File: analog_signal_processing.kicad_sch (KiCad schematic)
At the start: 62 parts, among them U3 PT2399, U4 CD4066BE, U5 PT2399, U8 TL072, U9 TL072

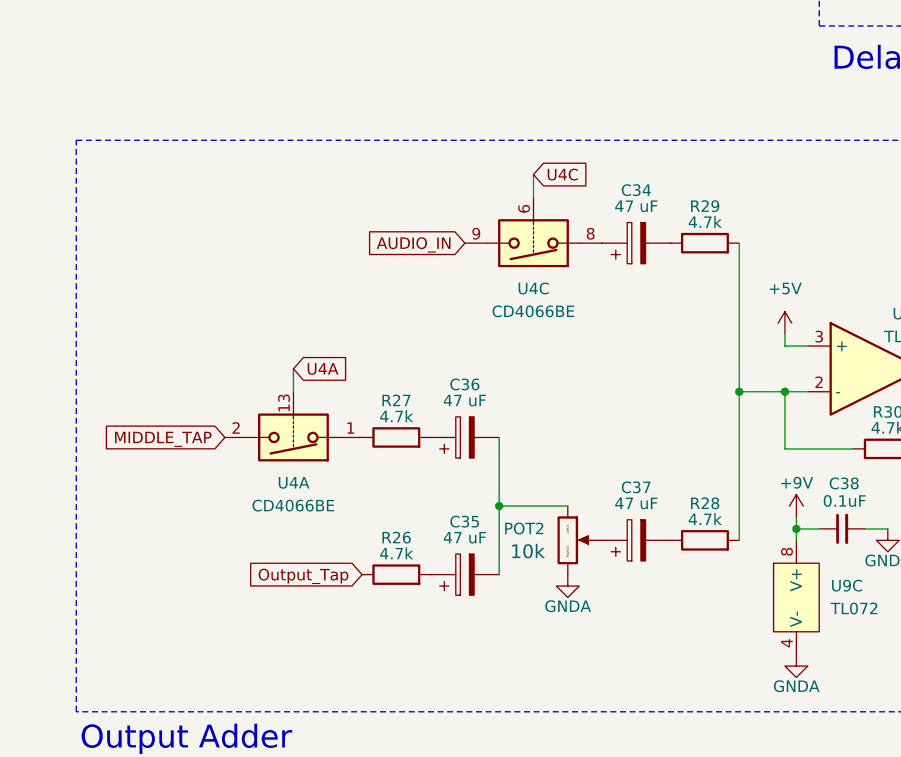
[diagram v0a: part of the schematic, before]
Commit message: wip on esp conns
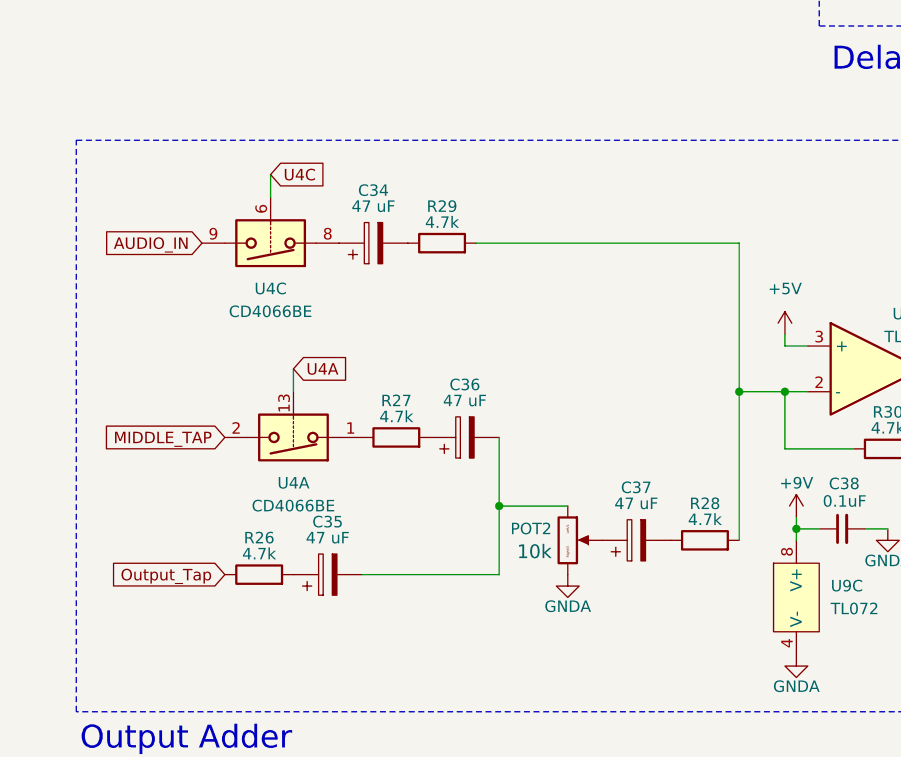
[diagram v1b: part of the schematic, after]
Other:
- moved on the sheet: C34, C35, R26, R29, U4C
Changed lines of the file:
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@@
 	(wire
 		(pts
+			(xy 63.5 172.72) (xy 63.5 165.1)
+		)
+		(stroke
+			(width 0)
+			(type default)
+		)
+	)
+	(wire
+		(pts
 			(xy 243.84 35.56) (xy 247.65 35.56)
 		)
@@
 	(wire
 		(pts
+			(xy 60.96 135.89) (xy 90.17 135.89)
+		)
+		(stroke
+			(width 0)
+			(type default)
+		)
+	)
+	(wire
+		(pts
 			(xy 198.12 54.61) (xy 198.12 55.88)
 		)
@@
 	(wire
 		(pts
-			(xy 67.31 128.27) (xy 67.31 130.81)
+			(xy 38.1 128.27) (xy 38.1 130.81)
 		)
 		(stroke
@@
 	(wire
 		(pts
-			(xy 95.25 146.05) (xy 95.25 147.32)
+			(xy 48.26 172.72) (xy 63.5 172.72)
 		)
 		(stroke
@@
 	(wire
 		(pts
-			(xy 198.12 16.51) (xy 198.12 19.05)
+			(xy 95.25 146.05) (xy 95.25 147.32)
 		)
 		(stroke
@@
 	(wire
 		(pts
-			(xy 138.43 83.82) (xy 138.43 85.09)
+			(xy 198.12 16.51) (xy 198.12 19.05)
 		)
 		(stroke
@@
 	(wire
 		(pts
-			(xy 154.94 31.75) (xy 160.02 31.75)
+			(xy 138.43 83.82) (xy 138.43 85.09)
 		)
 		(stroke
@@
 	(wire
 		(pts
-			(xy 107.95 33.02) (xy 107.95 41.91)
+			(xy 154.94 31.75) (xy 160.02 31.75)
 		)
 		(stroke
@@
 	(wire
 		(pts
-			(xy 63.5 165.1) (xy 63.5 172.72)
+			(xy 107.95 33.02) (xy 107.95 41.91)
 		)
 		(stroke
@@
 	(global_label "AUDIO_IN"
 		(shape input)
-		(at 59.69 135.89 180)
+		(at 30.48 135.89 180)
 		(fields_autoplaced yes)
 		(effects
@@
 		)
 		(property "Intersheetrefs" "${INTERSHEET_REFS}"
-			(at 48.1775 135.89 0)
+			(at 18.9675 135.89 0)
 			(effects
 				(font
@@
 	(global_label "U4C"
 		(shape input)
-		(at 67.31 128.27 0)
+		(at 38.1 128.27 0)
 		(fields_autoplaced yes)
 		(effects
@@
 		)
 		(property "Intersheetrefs" "${INTERSHEET_REFS}"
-			(at 74.1052 128.27 0)
+			(at 44.8952 128.27 0)
 			(effects
 				(font
@@
 	(global_label "Output_Tap"
 		(shape input)
-		(at 48.26 172.72 180)
+		(at 33.02 172.72 180)
 		(fields_autoplaced yes)
 		(effects
@@
 		)
 		(property "Intersheetrefs" "${INTERSHEET_REFS}"
-			(at 34.8127 172.72 0)
+			(at 19.5727 172.72 0)
 			(effects
 				(font
@@
 	(symbol
 		(lib_id "PCM_4ms_Resistor:4.7k_0603")
-		(at 86.36 135.89 90)
+		(at 57.15 135.89 90)
 		(unit 1)
 		(exclude_from_sim no)
@@
 		(dnp no)
 		(property "Reference" "R29"
-			(at 86.36 131.826 90)
+			(at 57.15 131.826 90)
 			(effects
 				(font
@@
 		)
 		(property "Value" "4.7k_0603"
-			(at 86.36 138.43 90)
+			(at 57.15 138.43 90)
 			(effects
 				(font
@@
 		)
 		(property "Footprint" "4ms_Resistor:R_0603"
-			(at 99.06 138.43 0)
+			(at 69.85 138.43 0)
 			(effects
 				(font
@@
 		)
 		(property "Datasheet" ""
-			(at 86.36 135.89 0)
+			(at 57.15 135.89 0)
 			(effects
 				(font
@@
 		)
 		(property "Description" "4k7, 1%, 1/10W, 0603"
-			(at 86.36 135.89 0)
+			(at 57.15 135.89 0)
 			(effects
 				(font
@@
 		)
 		(property "Specifications" "4k7, 1%, 1/10W, 0603"
-			(at 94.234 138.43 0)
+			(at 65.024 138.43 0)
 			(effects
 				(font
@@
 		)
 		(property "Manufacturer" "Yageo"
-			(at 95.758 138.43 0)
+			(at 66.548 138.43 0)
 			(effects
 				(font
@@
 		)
 		(property "Part Number" "RC0603FR-074K7L"
-			(at 97.282 138.43 0)
+			(at 68.072 138.43 0)
 			(effects
 				(font
@@
 		)
 		(property "Display" "4.7k"
-			(at 86.36 133.604 90)
+			(at 57.15 133.604 90)
 			(effects
 				(font
@@
 		)
 		(property "JLCPCB ID" "C23162"
-			(at 86.36 135.89 0)
+			(at 57.15 135.89 0)
 			(effects
 				(font
@@
 	(symbol
 		(lib_id "Device:C_Polarized")
-		(at 59.69 172.72 90)
+		(at 44.45 172.72 90)
 		(unit 1)
 		(exclude_from_sim no)
@@
 		(dnp no)
 		(property "Reference" "C35"
-			(at 59.69 166.878 90)
+			(at 44.45 166.878 90)
 			(effects
 				(font
@@
 		)
 		(property "Value" "47 uF"
-			(at 59.69 168.656 90)
+			(at 44.45 168.656 90)
 			(effects
 				(font
@@
 		)
 		(property "Footprint" ""
-			(at 63.5 171.7548 0)
+			(at 48.26 171.7548 0)
 			(effects
 				(font
@@
 		)
 		(property "Datasheet" "~"
-			(at 59.69 172.72 0)
+			(at 44.45 172.72 0)
 			(effects
 				(font
@@
 		)
 		(property "Description" "Polarized capacitor"
-			(at 59.69 172.72 0)
+			(at 44.45 172.72 0)
 			(effects
 				(font
@@
 		(on_board yes)
 		(dnp no)
-		(fields_autoplaced yes)
 		(property "Reference" "POT2"
-			(at 68.58 167.6399 0)
+			(at 69.342 167.64 0)
 			(effects
 				(font
@@
 		)
 		(property "Display" "10k"
-			(at 68.58 170.1799 0)
+			(at 69.342 170.18 0)
 			(effects
 				(font
@@
 	(symbol
 		(lib_id "PCM_4ms_Resistor:4.7k_0603")
-		(at 52.07 172.72 90)
+		(at 36.83 172.72 90)
 		(unit 1)
 		(exclude_from_sim no)
@@
 		(dnp no)
 		(property "Reference" "R26"
-			(at 52.07 168.656 90)
+			(at 36.83 168.656 90)
 			(effects
 				(font
@@
 		)
 		(property "Value" "4.7k_0603"
-			(at 52.07 175.26 90)
+			(at 36.83 175.26 90)
 			(effects
 				(font
@@
 		)
 		(property "Footprint" "4ms_Resistor:R_0603"
-			(at 64.77 175.26 0)
+			(at 49.53 175.26 0)
 			(effects
 				(font
@@
 		)
 		(property "Datasheet" ""
-			(at 52.07 172.72 0)
+			(at 36.83 172.72 0)
 			(effects
 				(font
@@
 		)
 		(property "Description" "4k7, 1%, 1/10W, 0603"
-			(at 52.07 172.72 0)
+			(at 36.83 172.72 0)
 			(effects
 				(font
@@
 		)
 		(property "Specifications" "4k7, 1%, 1/10W, 0603"
-			(at 59.944 175.26 0)
+			(at 44.704 175.26 0)
 			(effects
 				(font
@@
 		)
 		(property "Manufacturer" "Yageo"
-			(at 61.468 175.26 0)
+			(at 46.228 175.26 0)
 			(effects
 				(font
@@
 		)
 		(property "Part Number" "RC0603FR-074K7L"
-			(at 62.992 175.26 0)
+			(at 47.752 175.26 0)
 			(effects
 				(font
@@
 		)
 		(property "Display" "4.7k"
-			(at 52.07 170.434 90)
+			(at 36.83 170.434 90)
 			(effects
 				(font
@@
 		)
 		(property "JLCPCB ID" "C23162"
-			(at 52.07 172.72 0)
+			(at 36.83 172.72 0)
 			(effects
 				(font
@@
 	(symbol
 		(lib_id "Analog_Switch:CD4066BE")
-		(at 67.31 135.89 180)
+		(at 38.1 135.89 180)
 		(unit 3)
 		(exclude_from_sim no)
@@
 		(fields_autoplaced yes)
 		(property "Reference" "U4"
-			(at 67.31 140.97 0)
+			(at 38.1 140.97 0)
 			(effects
 				(font
@@
 		)
 		(property "Value" "CD4066BE"
-			(at 67.31 143.51 0)
+			(at 38.1 143.51 0)
 			(effects
 				(font
@@
 		)
 		(property "Footprint" "Package_DIP:DIP-14_W7.62mm"
-			(at 67.31 133.35 0)
+			(at 38.1 133.35 0)
 			(effects
 				(font
@@
 		)
 		(property "Datasheet" "https://www.ti.com/lit/ds/symlink/cd4066b.pdf"
-			(at 67.31 135.89 0)
+			(at 38.1 135.89 0)
 			(effects
 				(font
@@
 		)
 		(property "Description" "Quad 20V analog SPST 1:1 switch, DIP-14"
-			(at 67.31 135.89 0)
+			(at 38.1 135.89 0)
 			(effects
 				(font
@@
 	(symbol
 		(lib_id "Device:C_Polarized")
-		(at 78.74 135.89 90)
+		(at 49.53 135.89 90)
 		(unit 1)
 		(exclude_from_sim no)
@@
 		(dnp no)
 		(property "Reference" "C34"
-			(at 78.74 130.048 90)
+			(at 49.53 130.048 90)
 			(effects
 				(font
@@
 		)
 		(property "Value" "47 uF"
-			(at 78.74 131.826 90)
+			(at 49.53 131.826 90)
 			(effects
 				(font
@@
 		)
 		(property "Footprint" ""
-			(at 82.55 134.9248 0)
+			(at 53.34 134.9248 0)
 			(effects
 				(font
@@
 		)
 		(property "Datasheet" "~"
-			(at 78.74 135.89 0)
+			(at 49.53 135.89 0)
 			(effects
 				(font
@@
 		)
 		(property "Description" "Polarized capacitor"
-			(at 78.74 135.89 0)
+			(at 49.53 135.89 0)
 			(effects
 				(font

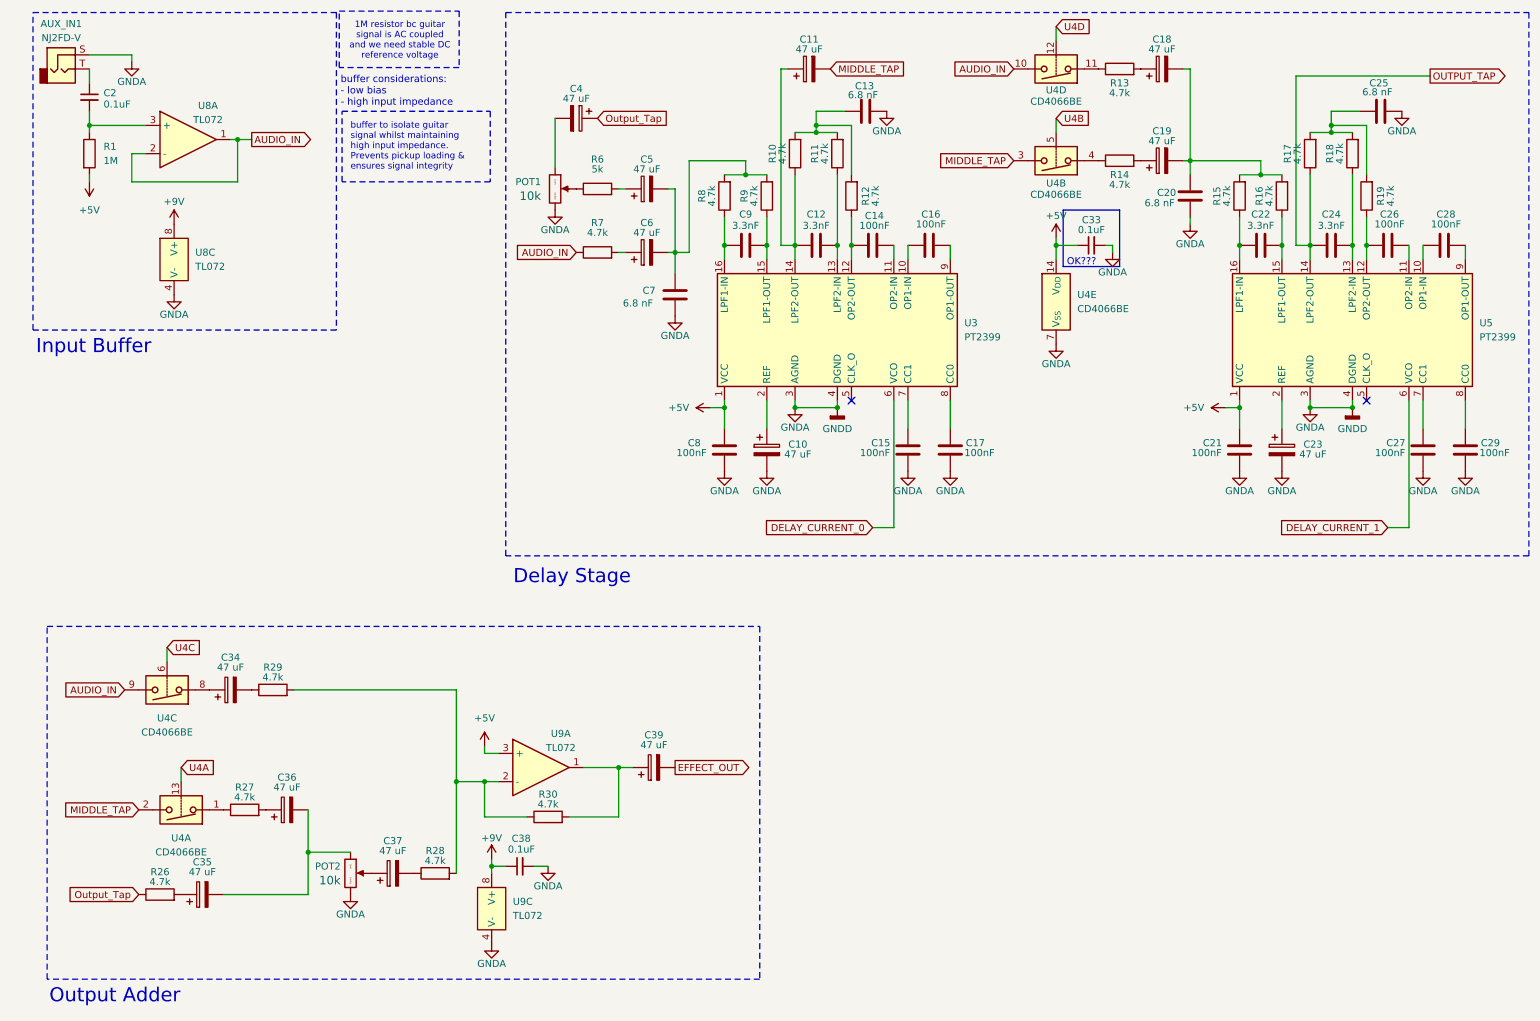
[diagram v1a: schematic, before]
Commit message: fixed a lot of things
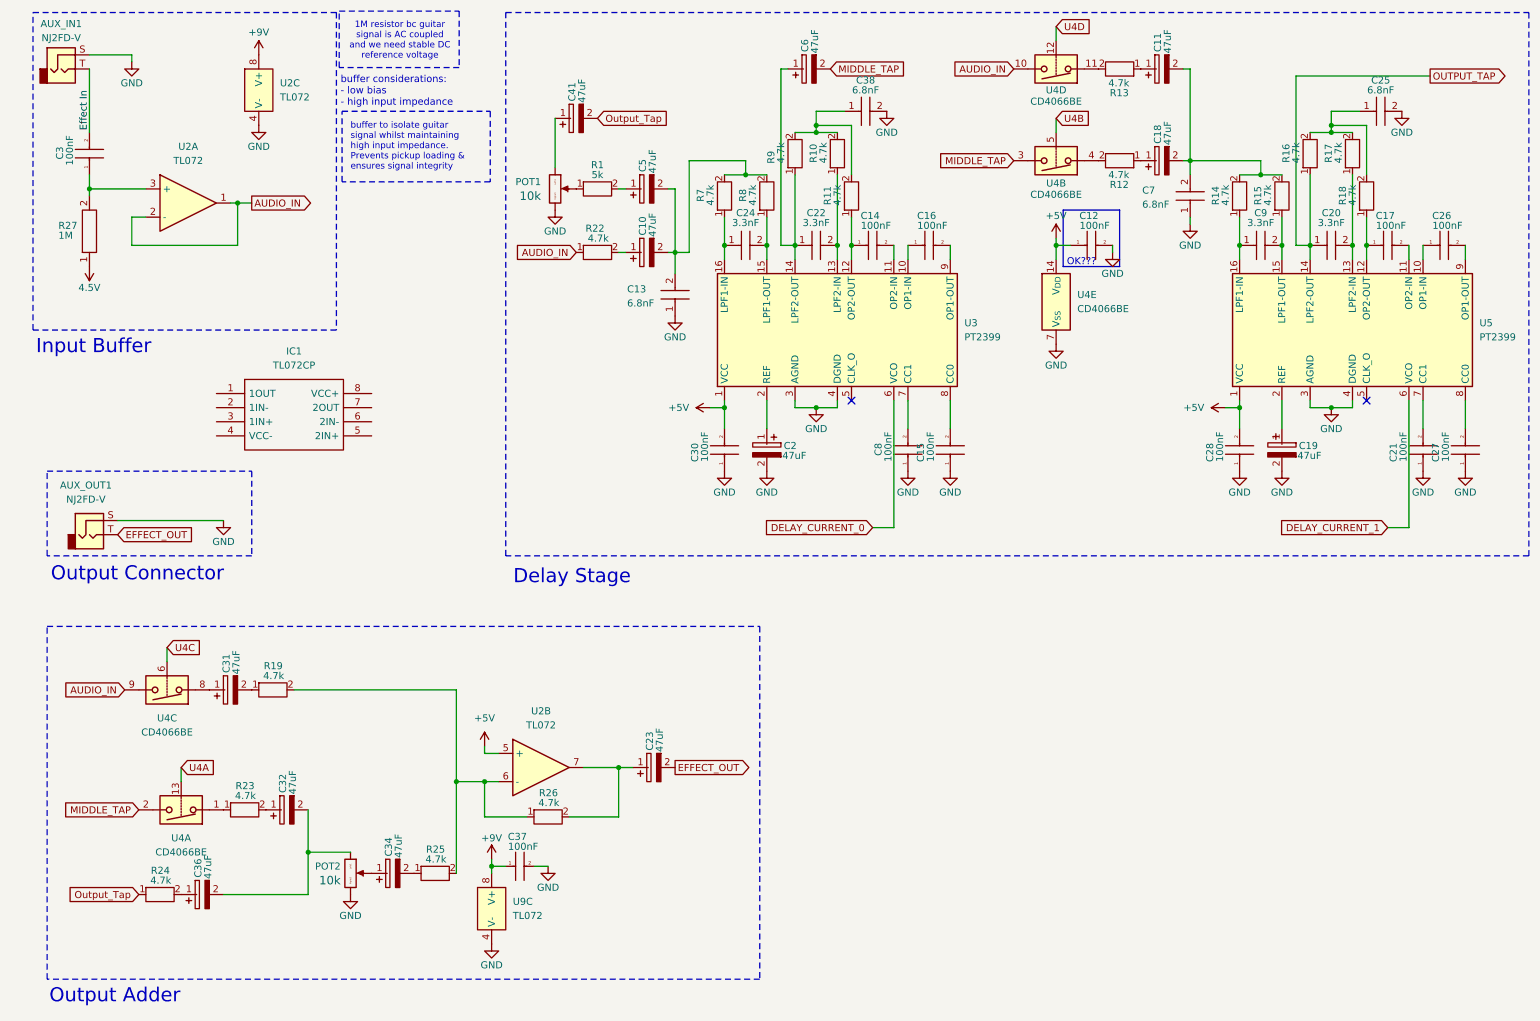
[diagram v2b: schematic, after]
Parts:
- removed C10, C11, C18, C19, C23, C34, C35, C36, C37, C39, C4, C5, C6: 47 uF, symbol Device:C_Polarized
- removed C12, C22, C24, C9: 3.3nF, symbol Device:C
- removed C13, C20, C25, C7: 6.8 nF, symbol Device:C
- removed C14, C15, C16, C17, C21, C26, C27, C28, C29, C8: 100nF, symbol Device:C
- removed C2, C33, C38: 100nF_0603_16V, 4ms_Capacitor:C_0603, symbol PCM_4ms_Capacitor:100nF_0603_16V
- removed R1: 1M, symbol Device:R
- removed R10, R11, R12, R13, R14, R15, R16, R17, R18, R19, R26, R27, R28, R29, R30, R7, R8, R9: 4.7k_0603, 4ms_Resistor:R_0603, symbol PCM_4ms_Resistor:4.7k_0603
- removed R6: 5k, symbol Device:R
- removed U8: TL072, 4ms_Package_SSOP:TSSOP-8_4.4x3mm_Pitch0.65mm, symbol PCM_4ms_IC:TL072
- removed unit 1 of U9
- added AUX_OUT1: NJ2FD-V, Connector_Audio:Jack_6.35mm_Neutrik_NJ2FD-V_Vertical, symbol Connector_Audio:NJ2FD-V
- added C10, C11, C18, C19, C2, C23, C31, C32, C34, C36, C41, C5, C6: 47uF, CAPPRD200W50D525H1250, symbol SamacSys_Parts:REA470M1CBK-0511P
- added C12, C14, C15, C16, C17, C21, C26, C27, C28, C3, C30, C37, C8: 100nF, SR211C104KARTR1, symbol SamacSys_Parts:SR211C104KARTR1
- added C13, C25, C38, C7: 6.8nF, SR211C682MARTR1, symbol SamacSys_Parts:SR211C682MARTR1
- added C20, C22, C24, C9: 3.3nF, RCER72A332K0DBH03A, symbol SamacSys_Parts:RCER72A332K0DBH03A
- added IC1: TL072CP, DIP794W53P254L959H508Q8N, symbol SamacSys_Parts:TL072CP
- added R1: 5k, RESAD1550W60L630D230, symbol SamacSys_Parts:YR1B4K99CC
- added R10, R11, R12, R13, R14, R15, R16, R17, R18, R19, R22, R23, R24, R25, R26, R7, R8, R9: 4.7k, RESAD1590W60L630D240, symbol SamacSys_Parts:MFR-25FRF52-4K7
- added R27: 1M, RESAD1590W60L630D240, symbol SamacSys_Parts:MFR-25FRF52-1M
- added U2: TL072, 4ms_Package_SSOP:TSSOP-8_4.4x3mm_Pitch0.65mm, symbol PCM_4ms_IC:TL072
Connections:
- net +5V: now also C12.1, C28.2, C30.2, U2.5 (+)
- net +9V: now also C37.1, U2.8 (V+)
- net AUDIO_IN: now also R22.1, U2.1, U2.2 (-)
- net EFFECT_OUT: now also AUX_OUT1.T, C23.2
- net MIDDLE_TAP: now also C6.2
- net OUTPUT_TAP: now also C20.1, R16.1
- net Output_Tap: now also C41.2, R24.1
- net at U3.15 (LPF1-OUT): now also C24.2, R8.1
- net at U5.10 (OP1-IN): now also C26.1
- net at U5.11 (OP2-IN): now also C17.2
- net at U5.12 (OP2-OUT): now also C17.1, R18.1
- net at U5.13 (LPF2-IN): now also C20.2, R17.1
- net at U5.15 (LPF1-OUT): now also C9.2, R15.1
- net at U5.16 (LPF1-IN): now also C9.1, R14.1
- net at U5.2 (REF): now also C19.1
- net at U5.7 (CC1): now also C21.2
- net at U5.8 (CC0): now also C27.2
- net at U5.9 (OP1-OUT): now also C26.2
- net at U3.16 (LPF1-IN): now also C24.1, R7.1
- net at U3.14 (LPF2-OUT): now also C22.1, C6.1, R9.1
- net Effect In: now reaches AUX_IN1.T
- net Effect In: now also C3.2
- net at POT2.1 (Left): now also C32.2, C36.2
- net at U4.1: now also R23.1
- net at U4.4: now also R12.2
- net at POT1.1 (Left): now also C41.1
- net at POT1.2 (Center): now also R1.1
- net at U4.11: now also R13.2
- net at POT2.2 (Center): now also C34.1
- net at U3.13 (LPF2-IN): now also C22.2, R10.1
- net at U3.12 (OP2-OUT): now also C14.1, R11.1
- net at U3.11 (OP2-IN): now also C14.2
- net at U4.8: now also C31.1
- net at U3.10 (OP1-IN): now also C16.1
- net at U3.9 (OP1-OUT): now also C16.2
- net at U3.7 (CC1): now also C8.2
- net at U3.8 (CC0): now also C15.2
- net at U3.2 (REF): now also C2.1
- net GNDA renamed GND
- net GND: now also AUX_OUT1.S, C12.2, C13.1, C15.1, C19.2, C2.2, C21.1, C25.2, C27.1, C28.1, C30.1, C37.2, C38.2, C7.1, C8.1, U2.4 (V-)
- new net: C36.1, R24.2
- new net: C34.2, R25.1
- new net: C3.1, R27.2, U2.3 (+)
- new net: C10.1, R22.2
- new net: R19.2, R25.2, R26.1, U2.6 (-)
- new net: C23.1, R26.2, U2.7
- new net: C18.1, R12.1
- new net: C31.2, R19.1
- new net: C10.2, C13.2, C5.2, R7.2, R8.2
- new net: C11.2, C18.2, C7.2, R14.2, R15.2
- new net: C25.1, R16.2, R17.2, R18.2
- new net: C38.1, R10.2, R11.2, R9.2
- new net: C11.1, R13.1
- new net: C5.1, R1.2
- new net: C32.1, R23.2
- new net 4.5V: R27.1
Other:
- note added: "Output Connector"
